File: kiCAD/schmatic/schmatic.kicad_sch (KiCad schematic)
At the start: 35 parts, among them J1 USB_C_Receptacle, J2 Conn_02x03_Counter_Clockwise, SW1 SW_MEC_5G, U1 STM32F401CBUx, U2 MPU-9250, U3 LP5907MFX-3.3, U4 USBLC6-2SC6, U5 XGZP6859D, Y1 16MHz, Y2 Crystal

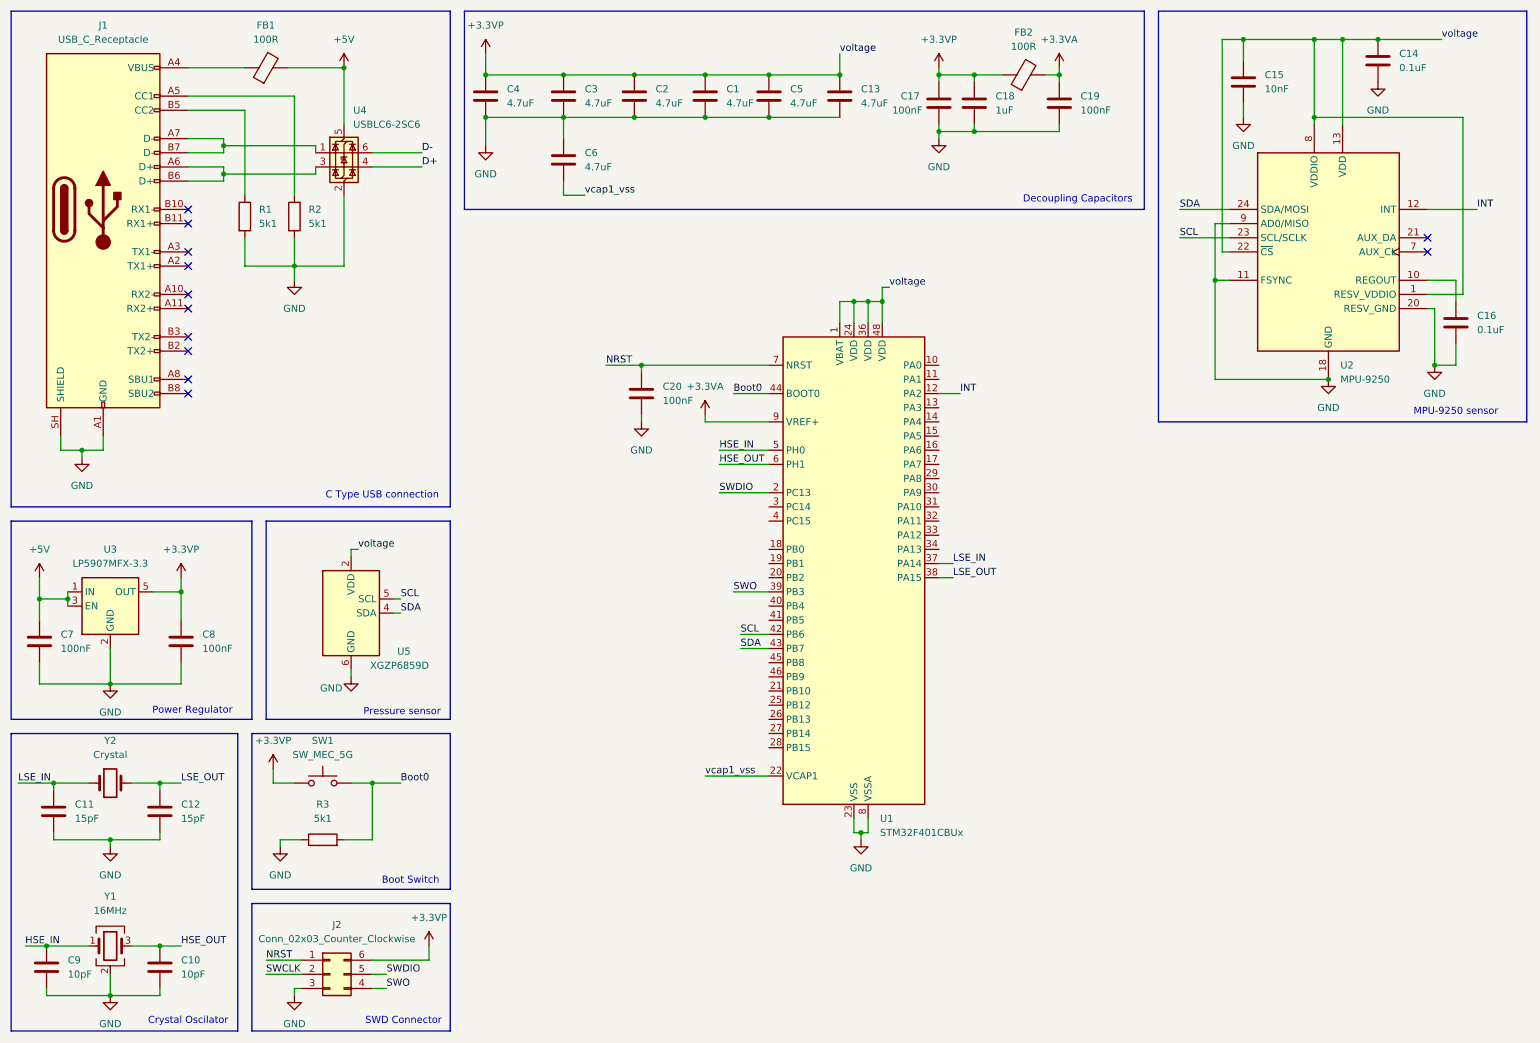
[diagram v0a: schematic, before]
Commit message: feat: PCB design finish
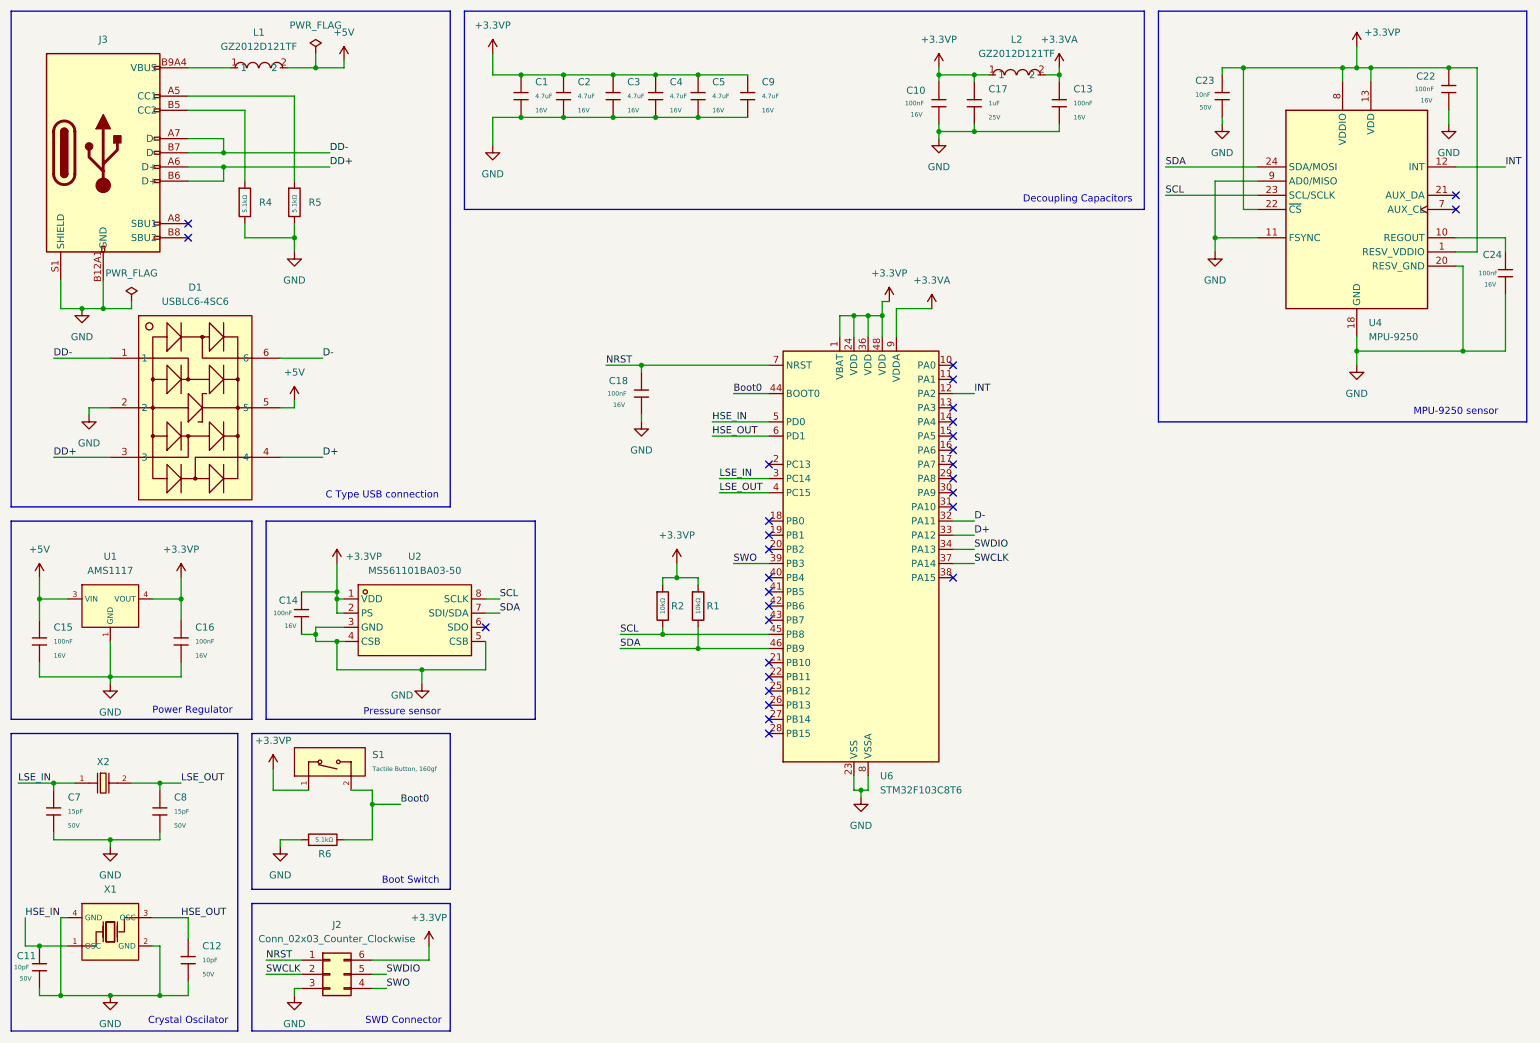
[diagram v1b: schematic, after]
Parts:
- removed C1, C13, C2, C3, C4, C5, C6: 4.7uF, symbol Device:C
- removed C10, C9: 10pF, symbol Device:C
- removed C11, C12: 15pF, symbol Device:C
- removed C14, C16: 0.1uF, symbol Device:C
- removed C15: 10nF, symbol Device:C
- removed C17, C19, C20, C7, C8: 100nF, symbol Device:C
- removed C18: 1uF, symbol Device:C
- removed FB1, FB2: 100R, symbol Device:FerriteBead
- removed J1: USB_C_Receptacle, symbol Connector:USB_C_Receptacle
- removed R1, R2, R3: 5k1, symbol Device:R
- removed SW1: SW_MEC_5G, Button_Switch_SMD:SW_MEC_5GSH9, symbol Switch:SW_MEC_5G
- removed U1: STM32F401CBUx, Package_DFN_QFN:QFN-48-1EP_7x7mm_P0.5mm_EP5.6x5.6mm, symbol MCU_ST_STM32F4:STM32F401CBUx
- removed U2: MPU-9250, Sensor_Motion:InvenSense_QFN-24_3x3mm_P0.4mm, symbol Sensor_Motion:MPU-9250
- removed U3: LP5907MFX-3.3, Package_TO_SOT_SMD:SOT-23-5, symbol Regulator_Linear:LP5907MFX-3.3
- removed U4: USBLC6-2SC6, Package_TO_SOT_SMD:SOT-23-6, symbol Power_Protection:USBLC6-2SC6
- removed U5: XGZP6859D, Sensor_Pressure:CFSensor_XGZP6859D_7x7mm, symbol Sensor_Pressure:XGZP6859D
- removed Y1: 16MHz, symbol Device:Crystal_GND24
- removed Y2: Crystal, symbol Device:Crystal
- added C1, C2, C3, C4, C5, C9: 4.7uF, PCM_JLCPCB:C_0603, symbol PCM_JLCPCB-Capacitors:0603,4.7uF
- added C10, C13, C14, C15, C16, C18, C22, C24: 100nF, PCM_JLCPCB:C_0402, symbol PCM_JLCPCB-Capacitors:0402,100nF
- added C11, C12: 10pF, PCM_JLCPCB:C_0402, symbol PCM_JLCPCB-Capacitors:0402,10pF
- added C17: 1uF, PCM_JLCPCB:C_0402, symbol PCM_JLCPCB-Capacitors:0402,1uF
- added C23: 10nF, PCM_JLCPCB:C_0402, symbol PCM_JLCPCB-Capacitors:0402,10nF
- added C7, C8: 15pF, PCM_JLCPCB:C_0402, symbol PCM_JLCPCB-Capacitors:0402,15pF
- added D1: USBLC6-4SC6, EasyEDA:SOT-23-6_L2.9-W1.6-P0.95-LS2.8-BL, symbol EasyEDA:USBLC6-4SC6
- added J3: Connector, USB-TYPE-C-16P, PCM_JLCPCB:TYPE-C-SMD_HX-TYPE-C-16PIN, symbol PCM_JLCPCB-Extended:Connector, USB-TYPE-C-16P
- added L1, L2: GZ2012D121TF, EasyEDA:L0805, symbol EasyEDA:GZ2012D121TF
- added R1, R2: 10kΩ, PCM_JLCPCB:R_0603, symbol PCM_JLCPCB-Resistors:0402,10kΩ
- added R4, R5, R6: 5.1kΩ, PCM_JLCPCB:R_0805, symbol PCM_JLCPCB-Resistors:0805,5.1kΩ
- added S1: Tactile Button, 160gf, PCM_JLCPCB:SW_TS-1088-AR02016, symbol PCM_JLCPCB-Connectors_Buttons:Tactile Button, 160gf, 12V, 50mA, 4.0mm
- added U1: AMS1117, PCM_JLCPCB:SOT-223-3_L6.5-W3.4-P2.30-LS7.0-BR, symbol PCM_JLCPCB-Power:LDO, 3.3V, 1A
- added U2: MS561101BA03-50, EasyEDA:SENSORS-SMD_MS5611-01BA03, symbol EasyEDA:MS561101BA03-50
- added U4: MPU-9250, Sensor_Motion:InvenSense_QFN-24_3x3mm_P0.4mm, symbol Sensor_Motion:MPU-9250
- added U6: STM32F103C8T6, PCM_JLCPCB:LQFP-48_7x7mm_P0.5mm, symbol PCM_JLCPCB-MCUs:STM32F103C8T6
- added X1: X322516MLB4SI, PCM_JLCPCB:OSC-SMD_4P-L3.2-W2.5-BL, symbol PCM_JLCPCB-Crystals:Crystal, 16MHz, 9pF
- added X2: Q13FC1350000400, PCM_JLCPCB:FC-135R_L3.2-W1.5, symbol PCM_JLCPCB-Crystals:Crystal, 32.768kHz, 13pF
- J2: footprint (none) -> Connector_PinHeader_1.27mm:PinHeader_2x03_P1.27mm_Vertical
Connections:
- net +3.3VA: now also C13.1, L2.2, U6.9 (VDDA)
- net +3.3VP: now also C1.1, C10.1, C14.1, C16.1, C17.1, C2.1, C22.1, C23.1, C3.1, C4.1, C5.1, C9.1, L2.1, R1.1, R2.1, S1.1 (A), U1.2 (VOUT), U1.4 (VOUT), U2.1 (VDD), U2.2 (PS), U4.1 (RESV_VDDIO), U4.13 (VDD), U4.22 (~{CS}), U4.8 (VDDIO), U6.1 (VBAT), U6.24 (VDD), U6.36 (VDD), U6.48 (VDD)
- net +5V: now also C15.1, D1.5, L1.2, U1.3 (VIN)
- net Boot0: now also R6.2, S1.2 (B), U6.44 (BOOT0)
- net D+: now also D1.4, U6.33 (PA12)
- net D-: now also D1.6, U6.32 (PA11)
- net GND: now also C1.2, C10.2, C11.2, C12.2, C13.2, C14.2, C15.2, C16.2, C17.2, C18.2, C2.2, C22.2, C23.2, C24.2, C3.2, C4.2, C5.2, C7.2, C8.2, C9.2, D1.2, J3.A12B1 (GND), J3.B12A1 (GND), J3.S1 (SHIELD), R4.2, R5.2, R6.1, U1.1 (GND), U2.3 (GND), U2.4 (CSB), U2.5 (CSB), U4.11 (FSYNC), U4.18 (GND), U4.20 (RESV_GND), U4.9 (AD0/MISO), U6.23 (VSS), U6.35 (VSS), U6.47 (VSS), U6.8 (VSSA), X1.2 (GND), X1.4 (GND)
- net HSE_IN: now also C11.1, U6.5 (PD0), X1.1 (OSC)
- net HSE_OUT: now also C12.1, U6.6 (PD1), X1.3 (OSC)
- net INT: now also U4.12 (INT), U6.12 (PA2)
- net LSE_IN: now also C7.1, U6.3 (PC14), X2.1
- net LSE_OUT: now also C8.1, U6.4 (PC15), X2.2
- net NRST: now also C18.1, U6.7 (NRST)
- net SCL: now also R2.2, U2.8 (SCLK), U4.23 (SCL/SCLK), U6.45 (PB8)
- net SDA: now also R1.2, U2.7 (SDI/SDA), U4.24 (SDA/MOSI), U6.46 (PB9)
- net SWCLK: now also U6.37 (PA14)
- net SWDIO: now also U6.34 (PA13)
- net SWO: now also U6.39 (PB3)
- new net: J3.A5 (CC1), R5.1
- new net: C24.1, U4.10 (REGOUT)
- new net: J3.A9B4 (VBUS), J3.B9A4 (VBUS), L1.1
- new net: J3.B5 (CC2), R4.1
- new net DD+: D1.3, J3.A6 (D+), J3.B6 (D+)
- new net DD-: D1.1, J3.A7 (D-), J3.B7 (D-)
- no-connect marks 12 -> 30
